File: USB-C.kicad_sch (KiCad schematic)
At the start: 31 parts, among them IC2 LM73100RPWR, IC5 TPS2557QDRBTQ1, J5 USB_C_Receptacle_USB2.0_16P, J9 USB_A, U2 TPD1E05U06DYA, U3 TPD1E05U06DYA

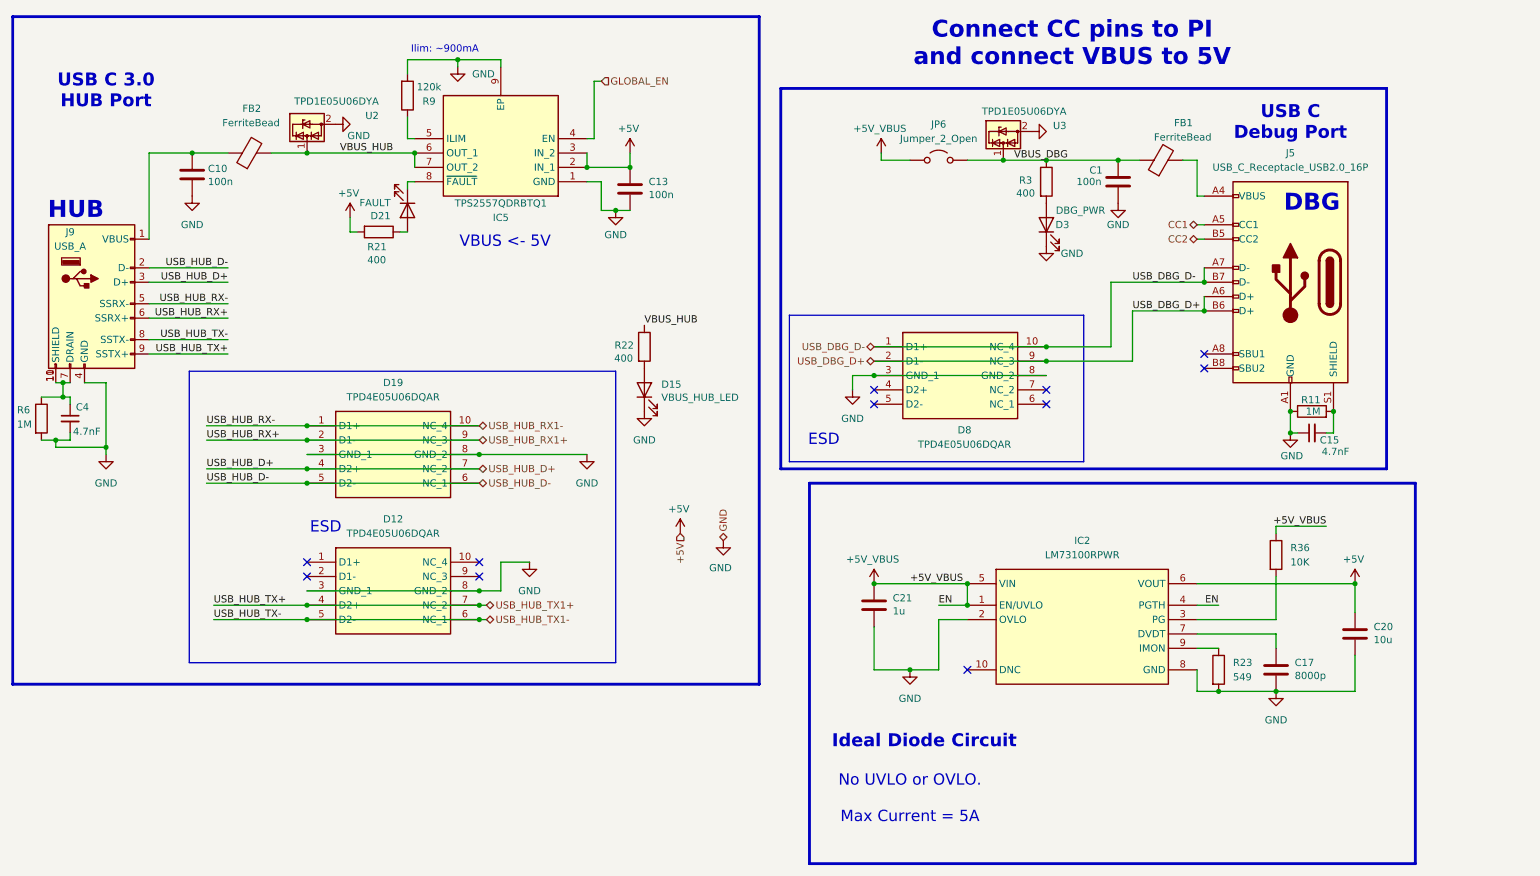
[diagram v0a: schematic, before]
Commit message: addressing mika's comments
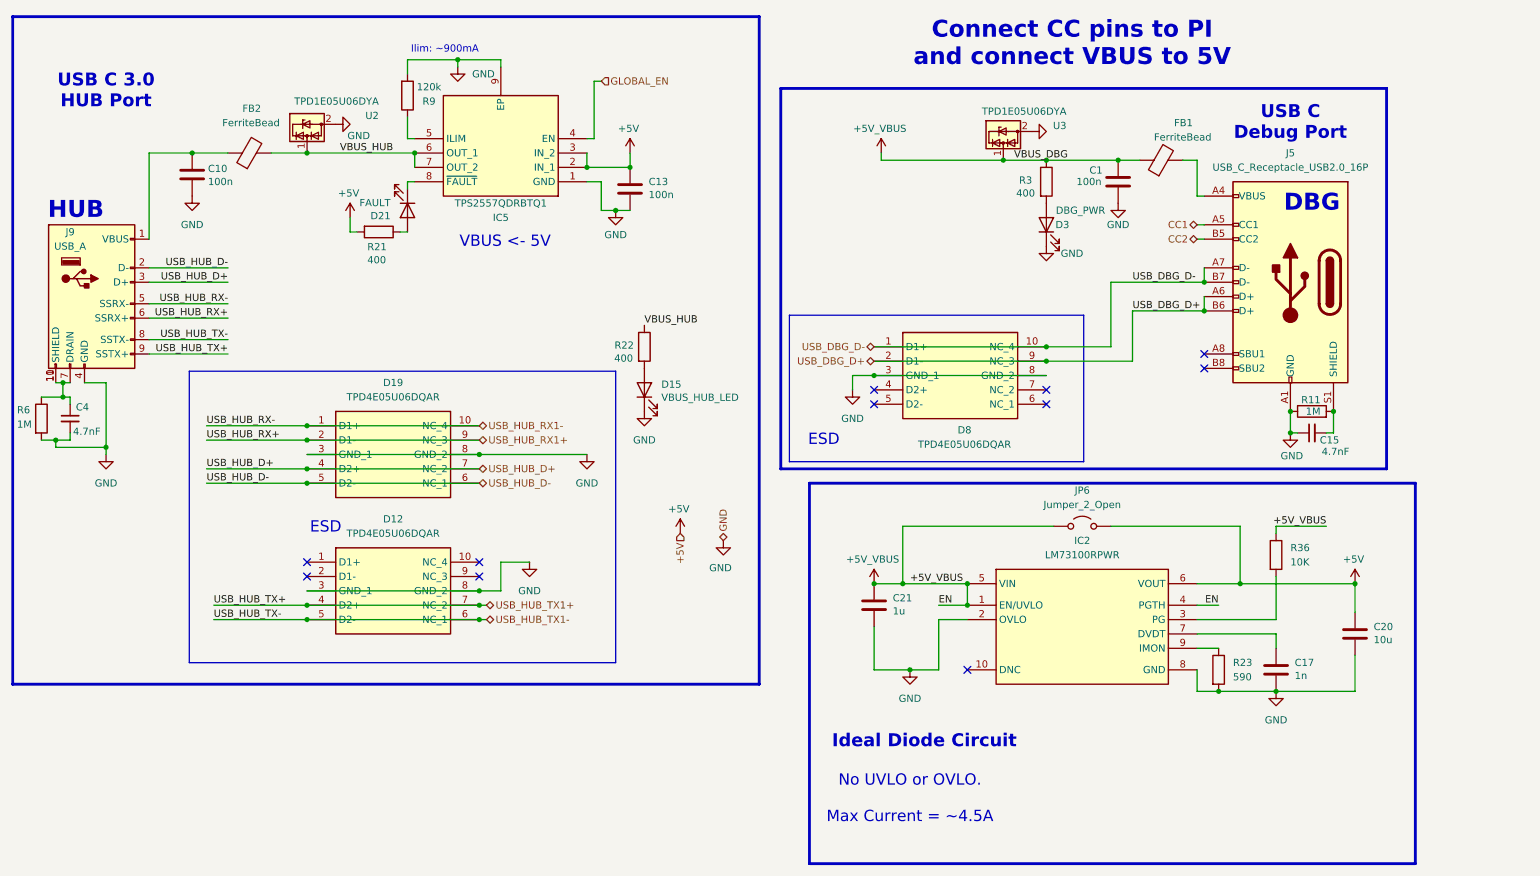
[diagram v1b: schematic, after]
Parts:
- C17: value 8000p -> 1n; JLC C14663 -> C1588; P/N MLASH168SB7104KTNA01 -> MLASU063SB7102KFNA01
- C20: footprint Capacitor_SMD:C_0603_1608Metric_Pad1.08x0.95mm_HandSolder -> Capacitor_SMD:C_0805_2012Metric_Pad1.18x1.45mm_HandSolder; JLC C14663 -> C440198; P/N MLASH168SB7104KTNA01 -> GRM21BR61H106KE43K
- C21: JLC C14663 -> C15849; P/N MLASH168SB7104KTNA01 -> MLASU168SB5105KTNA01
- R23: value 549 -> 590; JLC C5841024 -> C2076662; P/N PAT0603E4000BST1 -> CRCW0603590RFKEA
- R36: JLC C5841024 -> C25804; P/N PAT0603E4000BST1 -> CRCW060310K0FKEI
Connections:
- net +5V: now also JP6.2 (B)
- net +5V_VBUS: now also C1.1, FB1.1, R3.1, U3.1 (I/O)
- removed net VBUS_DBG: C1.1, FB1.1, JP6.2 (B), R3.1, U3.1 (I/O)
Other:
- note added: "No UVLO or OVLO. Max Current = ~4.5A"
- note removed: "No UVLO or OVLO. Max Current = 5A"
- moved on the sheet: JP6
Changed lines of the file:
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@@
 		)
 	)
-	(text "No UVLO or OVLO.\n\nMax Current = 5A\n"
+	(text "No UVLO or OVLO.\n\nMax Current = ~4.5A\n"
 		(exclude_from_sim no)
 		(at 173.99 153.67 0)
@@
 	)
 	(junction
+		(at 232.41 115.57)
+		(diameter 0)
+		(color 0 0 0 0)
+	)
+	(junction
 		(at 67.31 39.37)
 		(diameter 0)
@@
 	)
 	(junction
+		(at 172.72 115.57)
+		(diameter 0)
+		(color 0 0 0 0)
+	)
+	(junction
 		(at 167.64 115.57)
 		(diameter 0)
@@
 	(wire
 		(pts
-			(xy 184.15 40.64) (xy 190.5 40.64)
-		)
-		(stroke
-			(width 0)
-			(type default)
-		)
-	)
-	(wire
-		(pts
 			(xy 119.38 26.67) (xy 118.11 26.67)
 		)
@@
 	(wire
 		(pts
+			(xy 172.72 105.41) (xy 172.72 115.57)
+		)
+		(stroke
+			(width 0)
+			(type default)
+		)
+	)
+	(wire
+		(pts
 			(xy 31.75 80.01) (xy 31.75 91.44)
 		)
@@
 	(wire
 		(pts
+			(xy 199.39 105.41) (xy 172.72 105.41)
+		)
+		(stroke
+			(width 0)
+			(type default)
+		)
+	)
+	(wire
+		(pts
 			(xy 198.12 76.2) (xy 213.36 76.2)
 		)
@@
 	(wire
 		(pts
+			(xy 172.72 115.57) (xy 184.15 115.57)
+		)
+		(stroke
+			(width 0)
+			(type default)
+		)
+	)
+	(wire
+		(pts
 			(xy 242.57 88.9) (xy 241.3 88.9)
 		)
@@
 	(wire
 		(pts
+			(xy 232.41 115.57) (xy 252.73 115.57)
+		)
+		(stroke
+			(width 0)
+			(type default)
+		)
+	)
+	(wire
+		(pts
 			(xy 97.79 92.71) (xy 116.84 92.71)
 		)
@@
 	(wire
 		(pts
+			(xy 232.41 105.41) (xy 232.41 115.57)
+		)
+		(stroke
+			(width 0)
+			(type default)
+		)
+	)
+	(wire
+		(pts
 			(xy 101.6 22.86) (xy 101.6 24.13)
 		)
@@
 	(wire
 		(pts
-			(xy 224.79 115.57) (xy 252.73 115.57)
+			(xy 224.79 115.57) (xy 232.41 115.57)
 		)
 		(stroke
@@
 	(wire
 		(pts
+			(xy 209.55 105.41) (xy 232.41 105.41)
+		)
+		(stroke
+			(width 0)
+			(type default)
+		)
+	)
+	(wire
+		(pts
 			(xy 210.82 40.64) (xy 214.63 40.64)
 		)
@@
 	(wire
 		(pts
-			(xy 168.91 40.64) (xy 173.99 40.64)
+			(xy 168.91 40.64) (xy 190.5 40.64)
 		)
 		(stroke
@@
 	(wire
 		(pts
-			(xy 167.64 115.57) (xy 184.15 115.57)
+			(xy 167.64 115.57) (xy 172.72 115.57)
 		)
 		(stroke
@@
 			)
 		)
-		(property "Datasheet" "https://content.kemet.com/datasheets/KEM_C1002_X7R_SMD.pdf"
+		(property "Datasheet" ""
 			(at 167.64 119.38 0)
 			(effects
@@
 			)
 		)
-		(property "P/N" "MLASH168SB7104KTNA01 "
+		(property "P/N" "MLASU168SB5105KTNA01"
 			(at 167.64 119.38 0)
 			(effects
@@
 			)
 		)
-		(property "JLC" "C14663"
+		(property "JLC" "C15849"
 			(at 167.64 119.38 0)
 			(effects
@@
 			)
 		)
-		(property "Value" "8000p"
+		(property "Value" "1n"
 			(at 242.062 131.8514 0)
 			(effects
@@
 			)
 		)
-		(property "Datasheet" "https://content.kemet.com/datasheets/KEM_C1002_X7R_SMD.pdf"
+		(property "Datasheet" ""
 			(at 238.76 130.81 0)
 			(effects
@@
 			)
 		)
-		(property "P/N" "MLASH168SB7104KTNA01 "
+		(property "P/N" "MLASU063SB7102KFNA01"
 			(at 238.76 130.81 0)
 			(effects
@@
 			)
 		)
-		(property "JLC" "C14663"
+		(property "JLC" "C1588"
 			(at 238.76 130.81 0)
 			(effects
@@
 			)
 		)
-		(property "P/N" "PAT0603E4000BST1"
+		(property "P/N" "CRCW060310K0FKEI "
 			(at 238.76 110.49 0)
 			(effects
@@
 			)
 		)
-		(property "JLC" "C5841024"
+		(property "JLC" "C25804"
 			(at 238.76 110.49 0)
 			(effects
@@
 			)
 		)
-		(property "Value" "549"
+		(property "Value" "590"
 			(at 231.14 132.08 0)
 			(effects
@@
 			)
 		)
-		(property "P/N" "PAT0603E4000BST1"
+		(property "P/N" "CRCW0603590RFKEA"
 			(at 228.6 130.81 0)
 			(effects
@@
 			)
 		)
-		(property "JLC" "C5841024"
+		(property "JLC" "C2076662"
 			(at 228.6 130.81 0)
 			(effects
@@
 			)
 		)
-		(property "Footprint" "Capacitor_SMD:C_0603_1608Metric_Pad1.08x0.95mm_HandSolder"
+		(property "Footprint" "Capacitor_SMD:C_0805_2012Metric_Pad1.18x1.45mm_HandSolder"
 			(at 253.6952 128.27 0)
 			(effects
@@
 			)
 		)
-		(property "Datasheet" "https://content.kemet.com/datasheets/KEM_C1002_X7R_SMD.pdf"
+		(property "Datasheet" ""
 			(at 252.73 124.46 0)
 			(effects
@@
 			)
 		)
-		(property "P/N" "MLASH168SB7104KTNA01 "
+		(property "P/N" "GRM21BR61H106KE43K"
 			(at 252.73 124.46 0)
 			(effects
@@
 			)
 		)
-		(property "JLC" "C14663"
+		(property "JLC" "C440198"
 			(at 252.73 124.46 0)
 			(effects
@@
 	(symbol
 		(lib_id "Jumper:Jumper_2_Open")
-		(at 179.07 40.64 0)
+		(at 204.47 105.41 0)
 		(unit 1)
 		(exclude_from_sim no)
@@
 		(fields_autoplaced yes)
 		(property "Reference" "JP6"
-			(at 179.07 34.29 0)
+			(at 204.47 99.06 0)
 			(effects
 				(font
@@
 		)
 		(property "Value" "Jumper_2_Open"
-			(at 179.07 36.83 0)
+			(at 204.47 101.6 0)
 			(effects
 				(font
@@
 		)
 		(property "Footprint" "Connector_PinHeader_2.54mm:PinHeader_1x02_P2.54mm_Vertical"
-			(at 179.07 40.64 0)
+			(at 204.47 105.41 0)
 			(effects
 				(font
@@
 		)
 		(property "Datasheet" "~"
-			(at 179.07 40.64 0)
+			(at 204.47 105.41 0)
 			(effects
 				(font
@@
 		)
 		(property "Description" "Jumper, 2-pole, open"
-			(at 179.07 40.64 0)
+			(at 204.47 105.41 0)
 			(effects
 				(font
@@
 		)
 		(property "JLC" "N/A"
-			(at 179.07 40.64 0)
+			(at 204.47 105.41 0)
 			(effects
 				(font

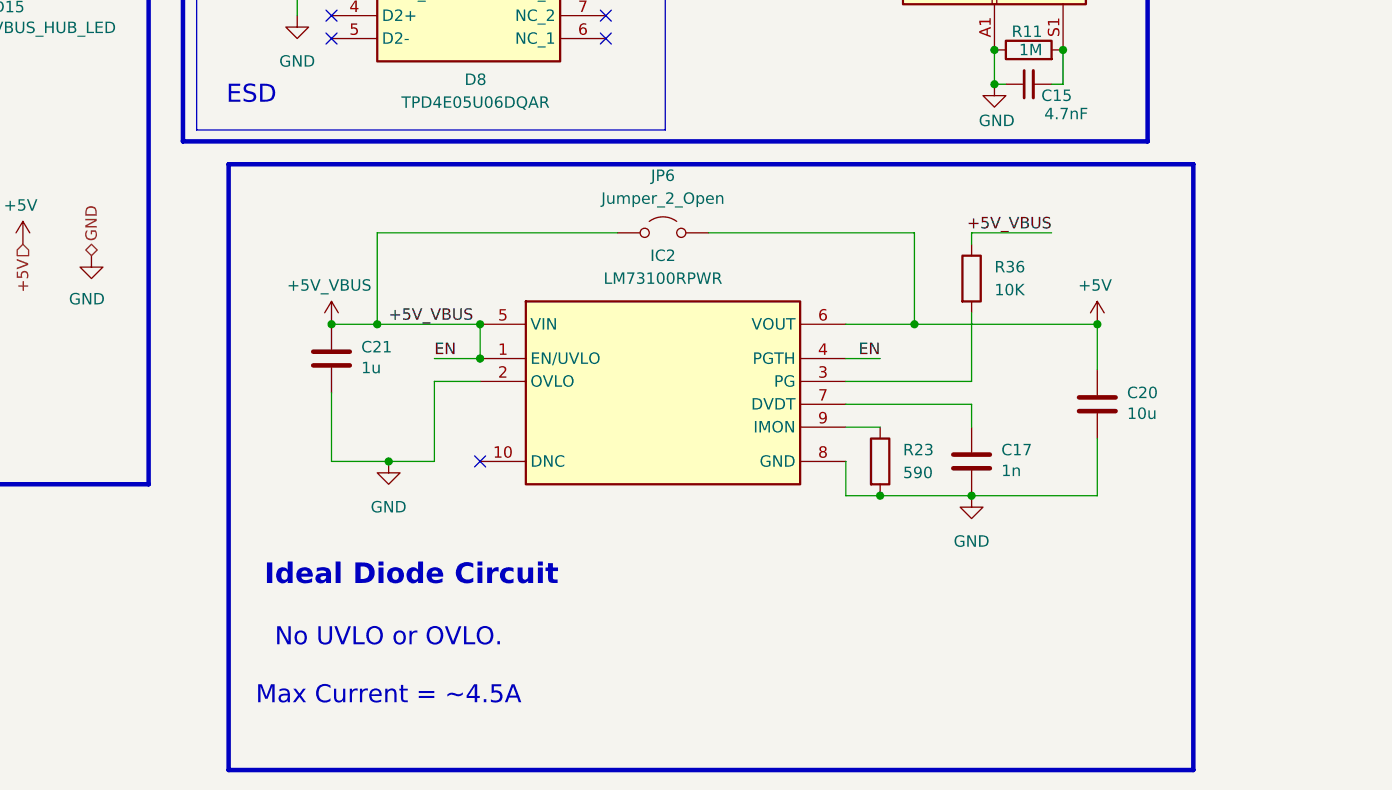
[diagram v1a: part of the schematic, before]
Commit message: mika changes
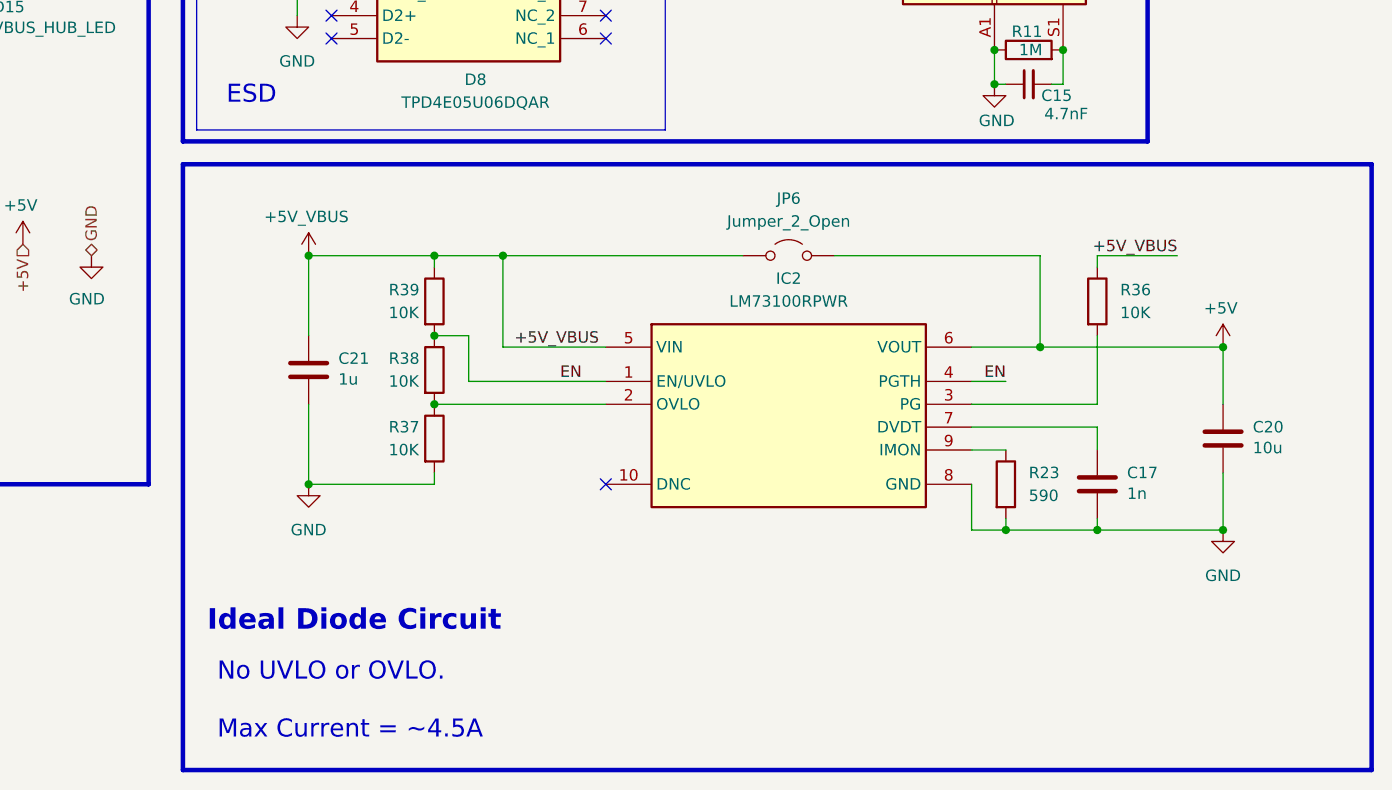
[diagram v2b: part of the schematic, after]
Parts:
- added R37, R38, R39: 10K, Resistor_SMD:R_0603_1608Metric_Pad0.98x0.95mm_HandSolder, symbol Device:R
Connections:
- net +5V_VBUS: now also R39.1; no longer IC2.1 (EN/UVLO), IC2.4 (PGTH)
- net GND: now also R37.2; no longer IC2.2 (OVLO)
- new net: IC2.2 (OVLO), R37.1, R38.2
- new net EN: IC2.1 (EN/UVLO), IC2.4 (PGTH), R38.1, R39.2
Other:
- moved on the sheet: C17, C20, C21, IC2, JP6, R23, R36

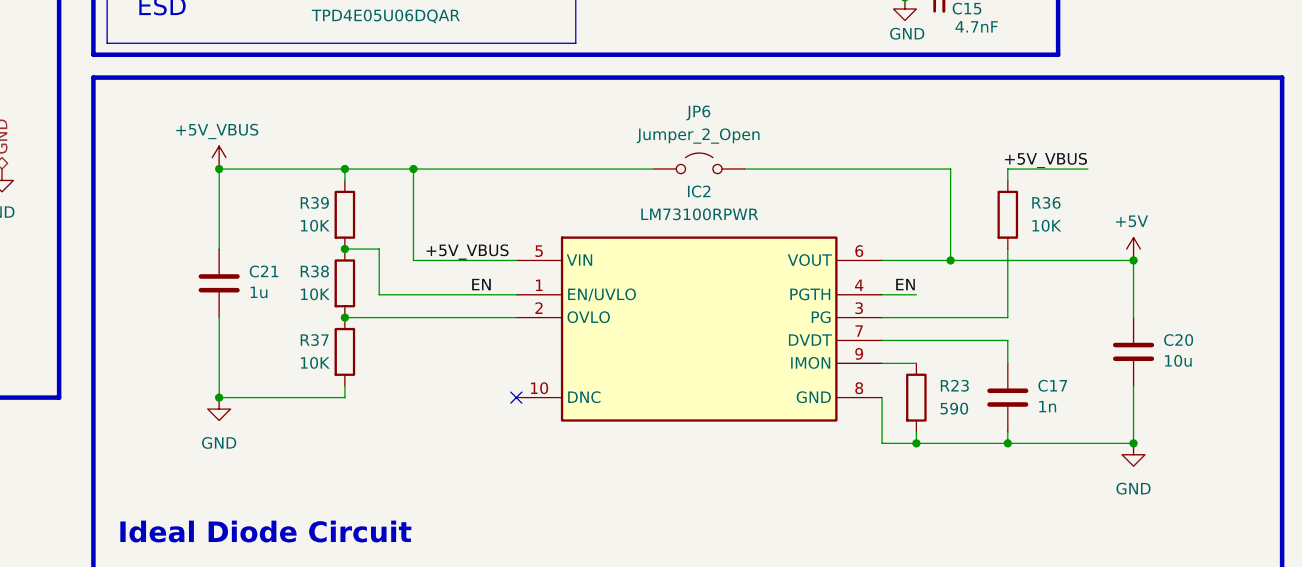
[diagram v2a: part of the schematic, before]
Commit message: mika changes
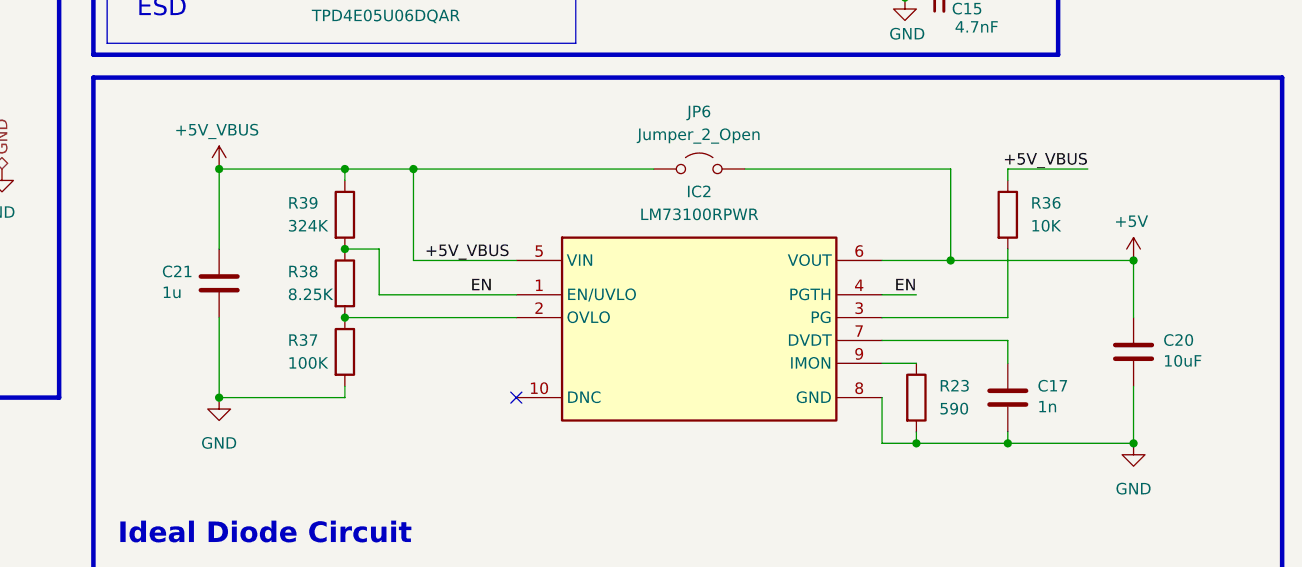
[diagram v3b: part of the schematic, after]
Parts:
- C20: value 10u -> 10uF
- R37: value 10K -> 100K; JLC (none) -> C25803; P/N (none) -> CRCW0603100KFKEE
- R38: value 10K -> 8.25K; JLC (none) -> C860536; P/N (none) -> RT0603BRB078K25L
- R39: value 10K -> 324K; JLC (none) -> C861321; P/N (none) -> RT0603BRD07324KL
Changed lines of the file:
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@@
 		(dnp no)
 		(property "Reference" "C21"
-			(at 168.402 119.38 0)
+			(at 158.75 119.38 0)
 			(effects
 				(font
@@
 		)
 		(property "Value" "1u"
-			(at 168.402 121.6914 0)
+			(at 158.75 121.6914 0)
 			(effects
 				(font
@@
 		(dnp no)
 		(property "Reference" "R39"
-			(at 173.99 111.76 0)
+			(at 172.72 111.76 0)
 			(effects
 				(font
@@
 			)
 		)
-		(property "Value" "10K"
-			(at 173.99 114.3 0)
+		(property "Value" "324K"
+			(at 172.72 114.3 0)
 			(effects
 				(font
@@
 			)
 		)
-		(property "P/N" ""
+		(property "P/N" "RT0603BRD07324KL"
 			(at 179.07 113.03 0)
 			(effects
@@
 			)
 		)
-		(property "JLC" ""
+		(property "JLC" "C861321"
 			(at 179.07 113.03 0)
 			(effects
@@
 		(dnp no)
 		(property "Reference" "R37"
-			(at 173.99 127 0)
+			(at 172.72 127 0)
 			(effects
 				(font
@@
 			)
 		)
-		(property "Value" "10K"
-			(at 173.99 129.54 0)
+		(property "Value" "100K"
+			(at 172.72 129.54 0)
 			(effects
 				(font
@@
 			)
 		)
-		(property "P/N" ""
+		(property "P/N" "CRCW0603100KFKEE"
 			(at 179.07 128.27 0)
 			(effects
@@
 			)
 		)
-		(property "JLC" ""
+		(property "JLC" "C25803"
 			(at 179.07 128.27 0)
 			(effects
@@
 		(dnp no)
 		(property "Reference" "R38"
-			(at 173.99 119.38 0)
+			(at 172.72 119.38 0)
 			(effects
 				(font
@@
 			)
 		)
-		(property "Value" "10K"
-			(at 173.99 121.92 0)
+		(property "Value" "8.25K"
+			(at 172.72 121.92 0)
 			(effects
 				(font
@@
 			)
 		)
-		(property "P/N" ""
+		(property "P/N" "RT0603BRB078K25L"
 			(at 179.07 120.65 0)
 			(effects
@@
 			)
 		)
-		(property "JLC" ""
+		(property "JLC" "C860536"
 			(at 179.07 120.65 0)
 			(effects
@@
 			)
 		)
-		(property "Value" "10u"
+		(property "Value" "10uF"
 			(at 270.002 129.3114 0)
 			(effects

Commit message: poop
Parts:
- IC2: JLC (none) -> C3210761
